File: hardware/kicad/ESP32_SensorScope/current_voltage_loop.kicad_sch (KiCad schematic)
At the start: 28 parts, among them Q1 PMOS, Q2 NMOS, Q7 NMOS, U18 OPA333xxDBV, U19 OPA333xxDBV, U20 OPA333xxDBV, U21 OPA333xxDBV, U22 ASSR-1218

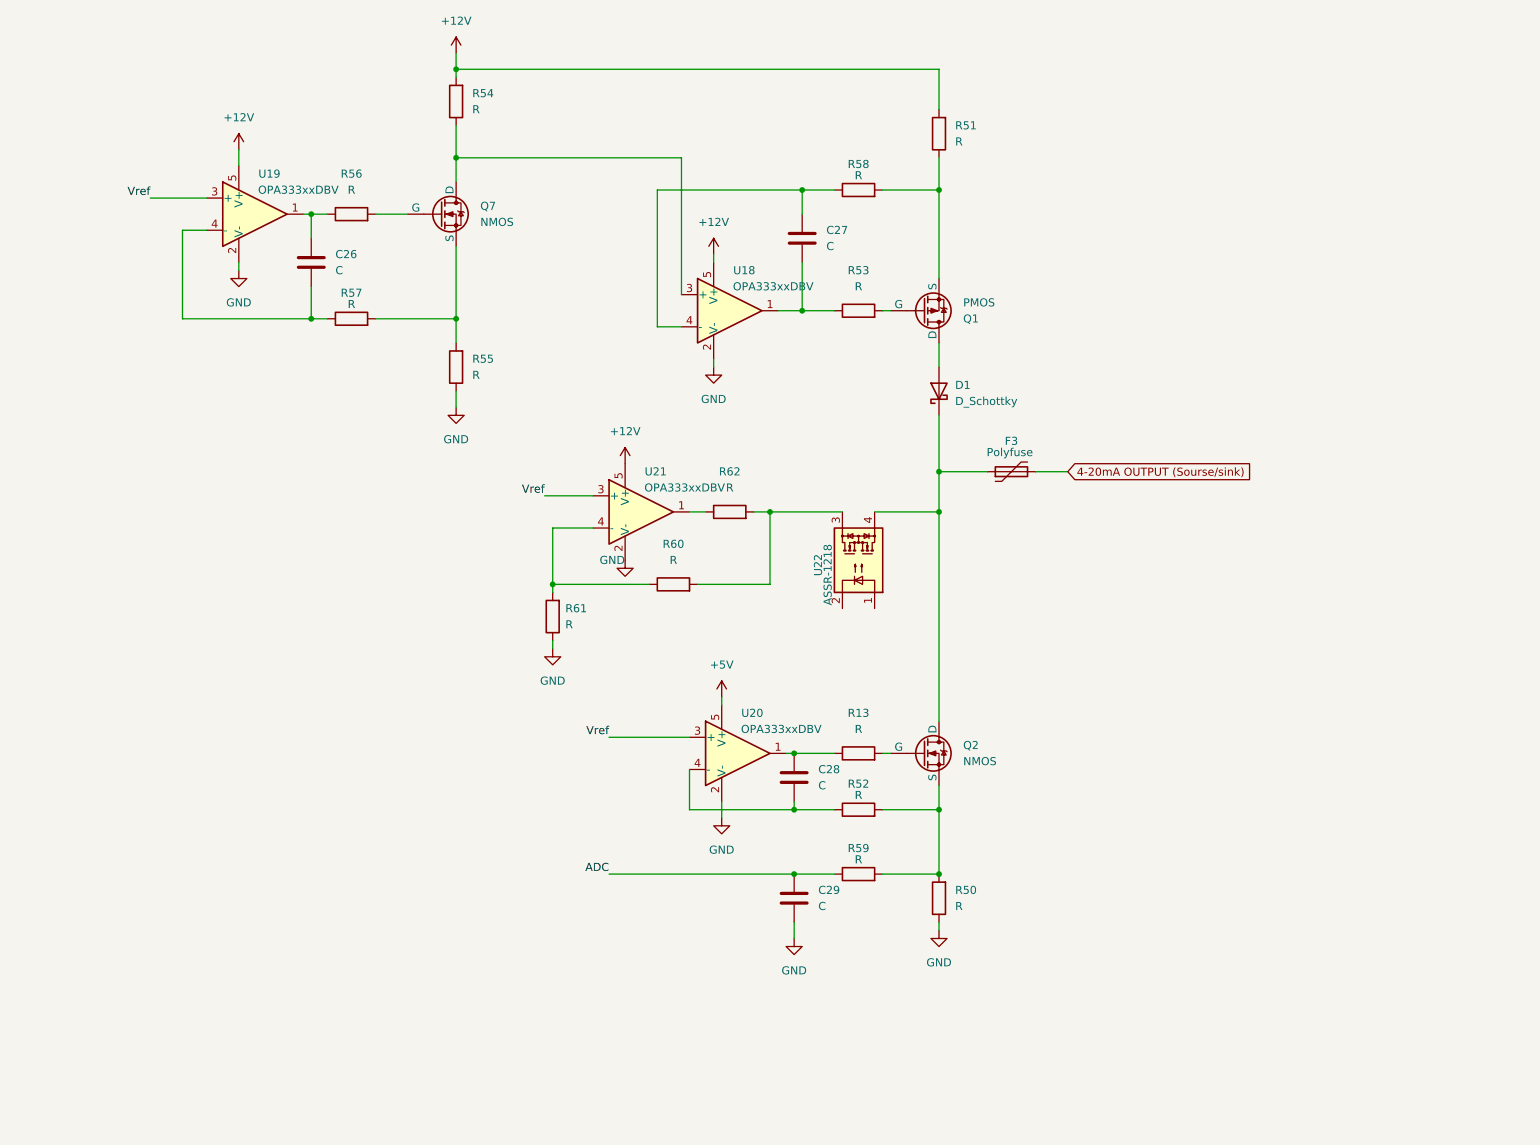
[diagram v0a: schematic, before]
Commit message: something probobly
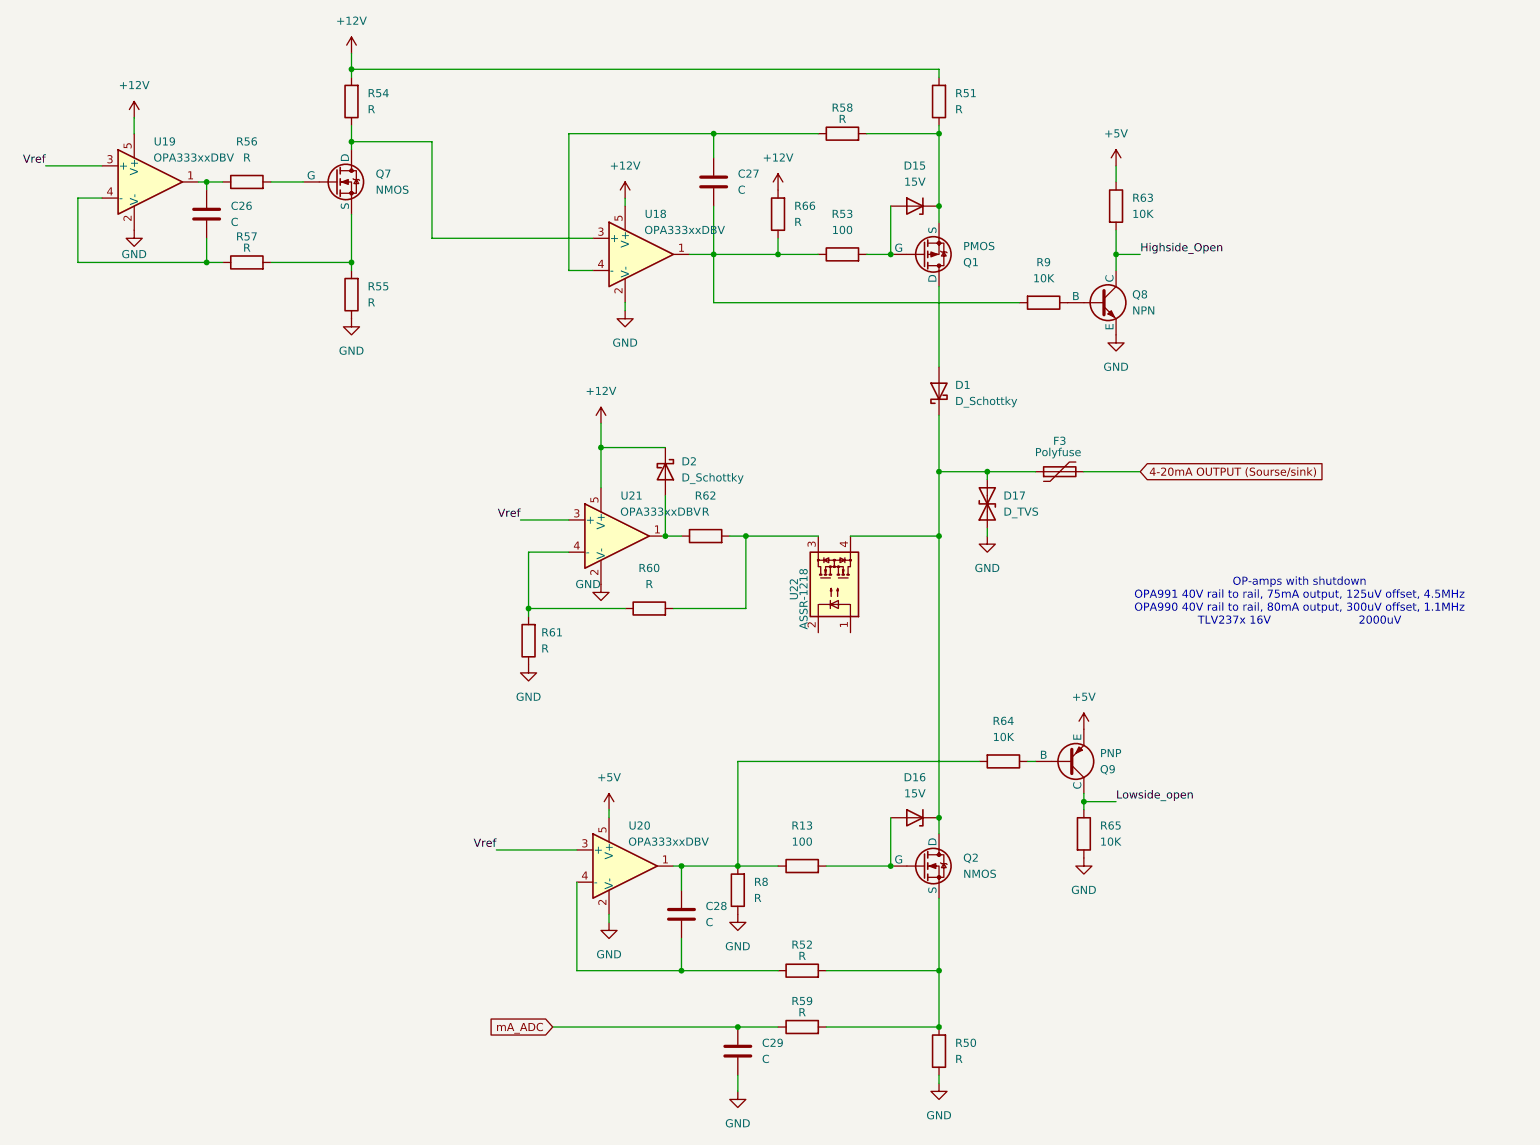
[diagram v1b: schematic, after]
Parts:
- added D15, D16: 15V, symbol Device:D_Zener
- added D17: D_TVS, symbol Device:D_TVS
- added D2: D_Schottky, symbol Device:D_Schottky
- added Q8: NPN, symbol Simulation_SPICE:NPN
- added Q9: PNP, symbol Simulation_SPICE:PNP
- added R63, R64, R65, R9: 10K, symbol Device:R
- added R66, R8: R, symbol Device:R
- R13, R53: value R -> 100
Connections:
- net +12V: now also D2.1 (K), R66.2
- net +5V: now also Q9.3 (E), R63.1
- net GND: now also D17.1 (A1), Q8.3 (E), R65.2, R8.1
- net at D1.1 (K), F3.1, Q2.1 (D)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: now also D16.1 (K), D17.2 (A2)
- net at Q2.2 (G), R13.2: now also D16.2 (A)
- net at Q1.3 (S), R51.1, R58.2: now also D15.1 (K)
- net at C27.2, R53.1, U18.1: now also R66.1, R9.2
- net at Q1.2 (G), R53.2: now also D15.2 (A)
- net at R62.1, U21.1: now also D2.2 (A)
- net at C28.1, R13.1, U20.1: now also R64.2, R8.2
- net ADC renamed mA_ADC
- new net: Q8.2 (B), R9.1
- new net: Q9.2 (B), R64.1
- new net Highside_Open: Q8.1 (C), R63.2
- new net Lowside_open: Q9.1 (C), R65.1
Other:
- note added: "OP-amps with shutdown OPA991 40V rail to rail, 75mA output, 125uV offset, 4.5MHz OPA990 40V rail to rail, 80mA output, 300uV offset, 1.1MHz TLV237x 16V 2000uV"
- moved on the sheet: C26, C27, C28, C29, F3, Q1, Q2, Q7, R13, R50, R51, R52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
